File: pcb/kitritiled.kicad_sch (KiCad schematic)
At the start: 15 parts, among them J1 ICSP, J2 ICSP, Q1 AO3401A, Q2 AO3400A, SW1 RESET, U1 PIC12LF1571-I/SN, U2 74LVC1G123

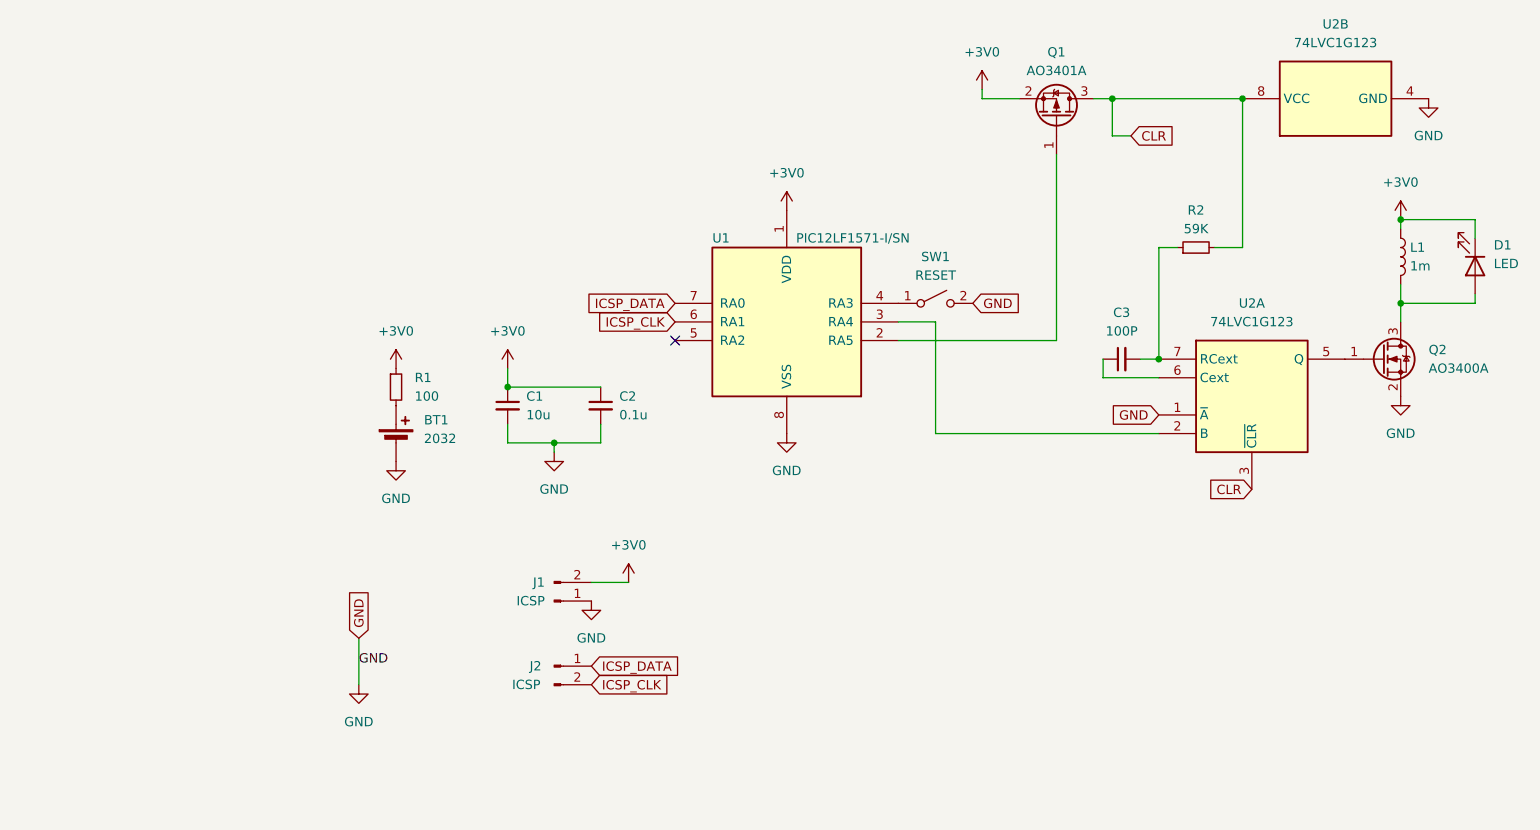
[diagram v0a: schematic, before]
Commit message: updates
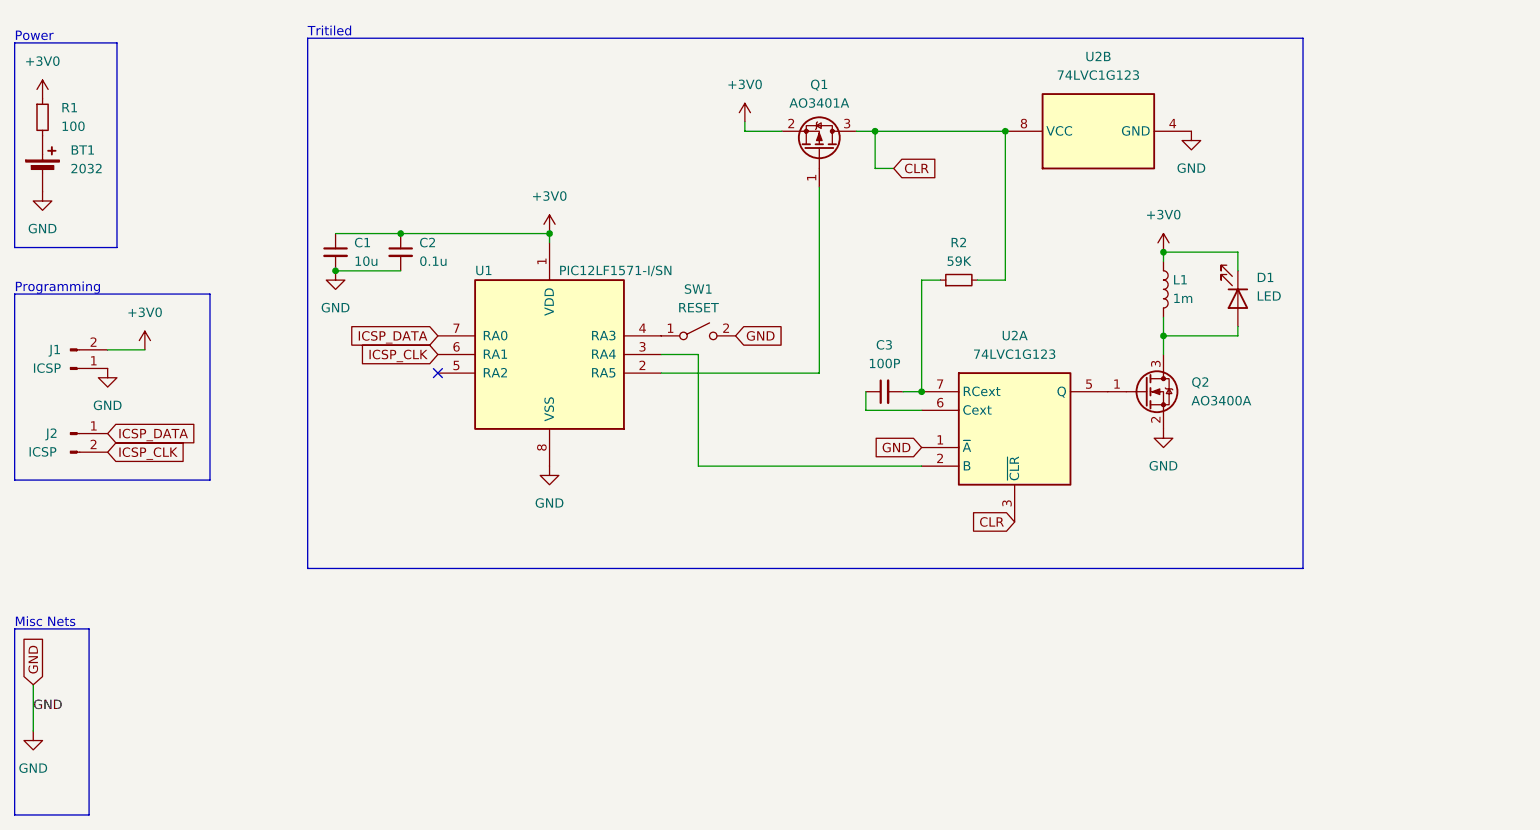
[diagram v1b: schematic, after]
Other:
- note added: "Misc Nets"
- note added: "Power"
- note added: "Programming"
- note added: "Tritiled"
- title: (none) -> KITRITILED
- moved on the sheet: BT1, C1, C2, C3, D1, J1, J2, L1, Q1, Q2, R1, R2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

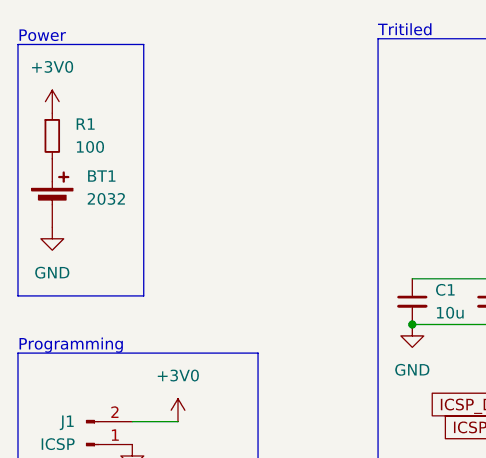
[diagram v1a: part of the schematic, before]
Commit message: prefab
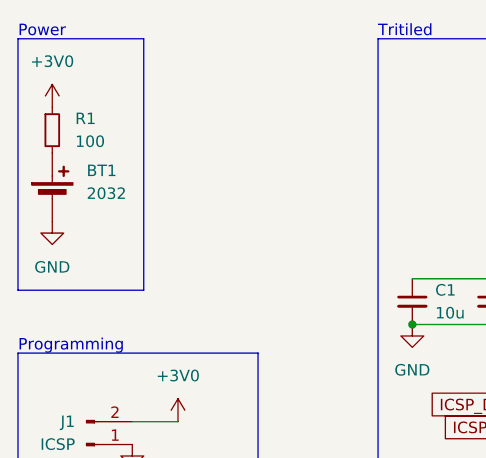
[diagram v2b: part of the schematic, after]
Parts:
- J1, J2: now left out of the parts list
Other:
- moved on the sheet: BT1, R1
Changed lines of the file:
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@@
     (fill (type none))
   )
-  (rectangle (start 16.51 17.78) (end 30.48 45.72)
+  (rectangle (start 16.51 17.145) (end 30.48 45.085)
     (stroke (width 0) (type default))
     (fill (type none))
@@
     (effects (font (size 1.27 1.27)) (justify left bottom))
   )
-  (text "Power" (at 16.51 17.78 0)
+  (text "Power" (at 16.51 17.145 0)
     (effects (font (size 1.27 1.27)) (justify left bottom))
   )
@@
     )
   )
-  (symbol (lib_id "Device:Battery_Cell") (at 20.32 35.56 0) (unit 1)
-    (in_bom yes) (on_board yes) (dnp no) (fields_autoplaced)
-    (property "Reference" "BT1" (at 24.13 32.4485 0)
-      (effects (font (size 1.27 1.27)) (justify left))
-    )
-    (property "Value" "2032" (at 24.13 34.9885 0)
-      (effects (font (size 1.27 1.27)) (justify left))
-    )
-    (property "Footprint" "Battery:BatteryHolder_LINX_BAT-HLD-012-SMT" (at 20.32 34.036 90)
-      (effects (font (size 1.27 1.27)) hide)
-    )
-    (property "Datasheet" "~" (at 20.32 34.036 90)
+  (symbol (lib_id "Device:Battery_Cell") (at 20.32 34.925 0) (unit 1)
+    (in_bom yes) (on_board yes) (dnp no) (fields_autoplaced)
+    (property "Reference" "BT1" (at 24.13 31.8135 0)
+      (effects (font (size 1.27 1.27)) (justify left))
+    )
+    (property "Value" "2032" (at 24.13 34.3535 0)
+      (effects (font (size 1.27 1.27)) (justify left))
+    )
+    (property "Footprint" "Battery:BatteryHolder_LINX_BAT-HLD-012-SMT" (at 20.32 33.401 90)
+      (effects (font (size 1.27 1.27)) hide)
+    )
+    (property "Datasheet" "~" (at 20.32 33.401 90)
       (effects (font (size 1.27 1.27)) hide)
     )
@@
   )
   (symbol (lib_id "Connector:Conn_01x02_Pin") (at 24.13 71.12 0) (unit 1)
-    (in_bom yes) (on_board yes) (dnp no)
+    (in_bom no) (on_board yes) (dnp no)
     (property "Reference" "J2" (at 21.59 71.12 0)
       (effects (font (size 1.27 1.27)))
@@
   )
   (symbol (lib_id "Connector:Conn_01x02_Pin") (at 24.13 62.23 0) (mirror x) (unit 1)
-    (in_bom yes) (on_board yes) (dnp no) (fields_autoplaced)
+    (in_bom no) (on_board yes) (dnp no) (fields_autoplaced)
     (property "Reference" "J1" (at 22.86 59.69 0)
       (effects (font (size 1.27 1.27)) (justify right))
@@
     )
   )
-  (symbol (lib_id "power:GND") (at 20.32 38.1 0) (unit 1)
-    (in_bom yes) (on_board yes) (dnp no) (fields_autoplaced)
-    (property "Reference" "#PWR06" (at 20.32 44.45 0)
-      (effects (font (size 1.27 1.27)) hide)
-    )
-    (property "Value" "GND" (at 20.32 43.18 0)
-      (effects (font (size 1.27 1.27)))
-    )
-    (property "Footprint" "" (at 20.32 38.1 0)
-      (effects (font (size 1.27 1.27)) hide)
-    )
-    (property "Datasheet" "" (at 20.32 38.1 0)
+  (symbol (lib_id "power:GND") (at 20.32 37.465 0) (unit 1)
+    (in_bom yes) (on_board yes) (dnp no) (fields_autoplaced)
+    (property "Reference" "#PWR06" (at 20.32 43.815 0)
+      (effects (font (size 1.27 1.27)) hide)
+    )
+    (property "Value" "GND" (at 20.32 42.545 0)
+      (effects (font (size 1.27 1.27)))
+    )
+    (property "Footprint" "" (at 20.32 37.465 0)
+      (effects (font (size 1.27 1.27)) hide)
+    )
+    (property "Datasheet" "" (at 20.32 37.465 0)
       (effects (font (size 1.27 1.27)) hide)
     )
@@
     )
   )
-  (symbol (lib_id "power:+3V0") (at 20.32 25.4 0) (unit 1)
-    (in_bom yes) (on_board yes) (dnp no) (fields_autoplaced)
-    (property "Reference" "#PWR01" (at 20.32 29.21 0)
-      (effects (font (size 1.27 1.27)) hide)
-    )
-    (property "Value" "+3V0" (at 20.32 20.32 0)
-      (effects (font (size 1.27 1.27)))
-    )
-    (property "Footprint" "" (at 20.32 25.4 0)
-      (effects (font (size 1.27 1.27)) hide)
-    )
-    (property "Datasheet" "" (at 20.32 25.4 0)
+  (symbol (lib_id "power:+3V0") (at 20.32 24.765 0) (unit 1)
+    (in_bom yes) (on_board yes) (dnp no) (fields_autoplaced)
+    (property "Reference" "#PWR01" (at 20.32 28.575 0)
+      (effects (font (size 1.27 1.27)) hide)
+    )
+    (property "Value" "+3V0" (at 20.32 19.685 0)
+      (effects (font (size 1.27 1.27)))
+    )
+    (property "Footprint" "" (at 20.32 24.765 0)
+      (effects (font (size 1.27 1.27)) hide)
+    )
+    (property "Datasheet" "" (at 20.32 24.765 0)
       (effects (font (size 1.27 1.27)) hide)
     )
@@
     )
   )
-  (symbol (lib_id "Device:R_Small") (at 20.32 27.94 0) (unit 1)
-    (in_bom yes) (on_board yes) (dnp no) (fields_autoplaced)
-    (property "Reference" "R1" (at 22.86 26.67 0)
-      (effects (font (size 1.27 1.27)) (justify left))
-    )
-    (property "Value" "100" (at 22.86 29.21 0)
-      (effects (font (size 1.27 1.27)) (justify left))
-    )
-    (property "Footprint" "Resistor_SMD:R_0402_1005Metric" (at 20.32 27.94 0)
-      (effects (font (size 1.27 1.27)) hide)
-    )
-    (property "Datasheet" "~" (at 20.32 27.94 0)
-      (effects (font (size 1.27 1.27)) hide)
-    )
-    (property "LCSC" "C25076" (at 20.32 27.94 0)
-      (effects (font (size 1.27 1.27)) hide)
-    )
+  (symbol (lib_id "Device:R_Small") (at 20.32 27.305 0) (unit 1)
+    (in_bom yes) (on_board yes) (dnp no) (fields_autoplaced)
+    (property "Reference" "R1" (at 22.86 26.035 0)
+      (effects (font (size 1.27 1.27)) (justify left))
+    )
+    (property "Value" "100" (at 22.86 28.575 0)
+      (effects (font (size 1.27 1.27)) (justify left))
+    )
+    (property "Footprint" "Resistor_SMD:R_0402_1005Metric" (at 20.32 27.305 0)
+      (effects (font (size 1.27 1.27)) hide)
+    )
+    (property "Datasheet" "~" (at 20.32 27.305 0)
+      (effects (font (size 1.27 1.27)) hide)
+    )
+    (property "LCSC" "C25076" (at 20.32 27.305 0)
+      (effects (font (size 1.27 1.27)) hide)
+    )
